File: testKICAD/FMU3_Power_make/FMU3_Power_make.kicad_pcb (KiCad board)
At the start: 2 copper layers, 17.5 x 10.5 mm, 13 parts, among them J1 Conn_01x03_Male, J2 Conn_01x04_Female, U1 MIC5332-SSYMT-TR

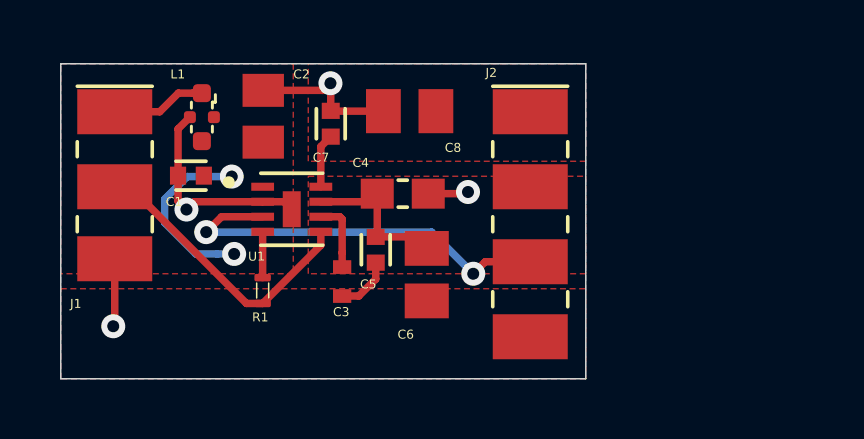
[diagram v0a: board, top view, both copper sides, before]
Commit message: Parts 3D modelling
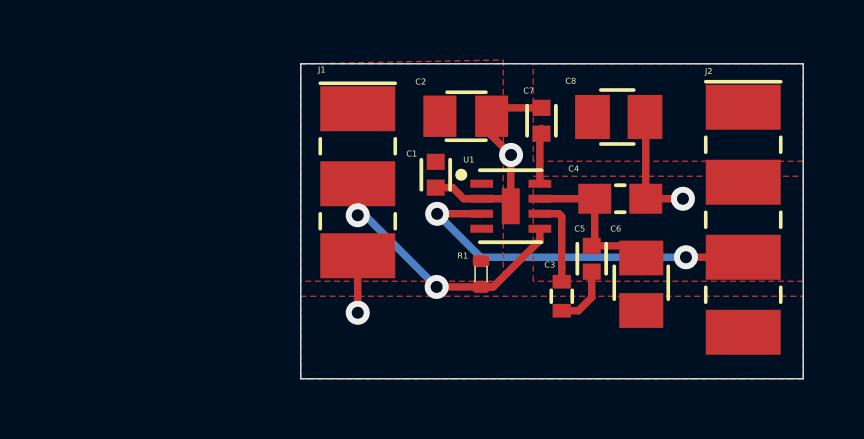
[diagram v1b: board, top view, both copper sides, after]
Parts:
- removed L1: Kyocera KNH16C104bA5TS EMI filter, woos_FMU3:KNH16C104DA5TS_Filter
- moved R1 9.32 mm to (107.5, 56.5)
- moved C1 8.16 mm to (106.0, 53.2), turned to 270 degrees
- moved J1 8.10 mm to (101.7, 49.9)
- moved C3 7.34 mm to (110.2, 57.2)
- moved U1 7.30 mm to (108.5, 54.2)
- moved C4 7.25 mm to (112.2, 54.0)
- moved C5 7.21 mm to (111.2, 56.0)
- moved C6 7.16 mm to (112.8, 56.9)
- moved J2 7.10 mm to (114.7, 49.9)
- moved C7 7.03 mm to (109.5, 51.4)
- moved C8 6.97 mm to (112.1, 51.3), turned to 0 degrees
- moved C2 6.75 mm to (107.0, 51.2), turned to 0 degrees
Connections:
- J1 pad 1: /VDD_5V_IN -> /FMU-VDD_5V5
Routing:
- net /FMU-VDD_5V5: track 7.61 -> 0.00 mm, vias 2 -> 0
- net /VDD_5V_IN: track 3.16 -> 0.00 mm
- net GND: track 17.6 -> 15.7 mm, vias 4 -> 3
- net /FMU-!RESET: track 13.6 -> 12.3 mm
- net Net-(C3-Pad1): track 2.34 -> 2.94 mm
- net /VDD_3V3_SENSORS_EN: track 9.73 -> 9.14 mm, vias 0 -> 2
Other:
- board size 17.5 x 10.5 mm -> 16.8 x 10.5 mm
